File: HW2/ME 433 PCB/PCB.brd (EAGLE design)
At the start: 50 x 50 mm, 22 parts, among them J1 USB-MB-H

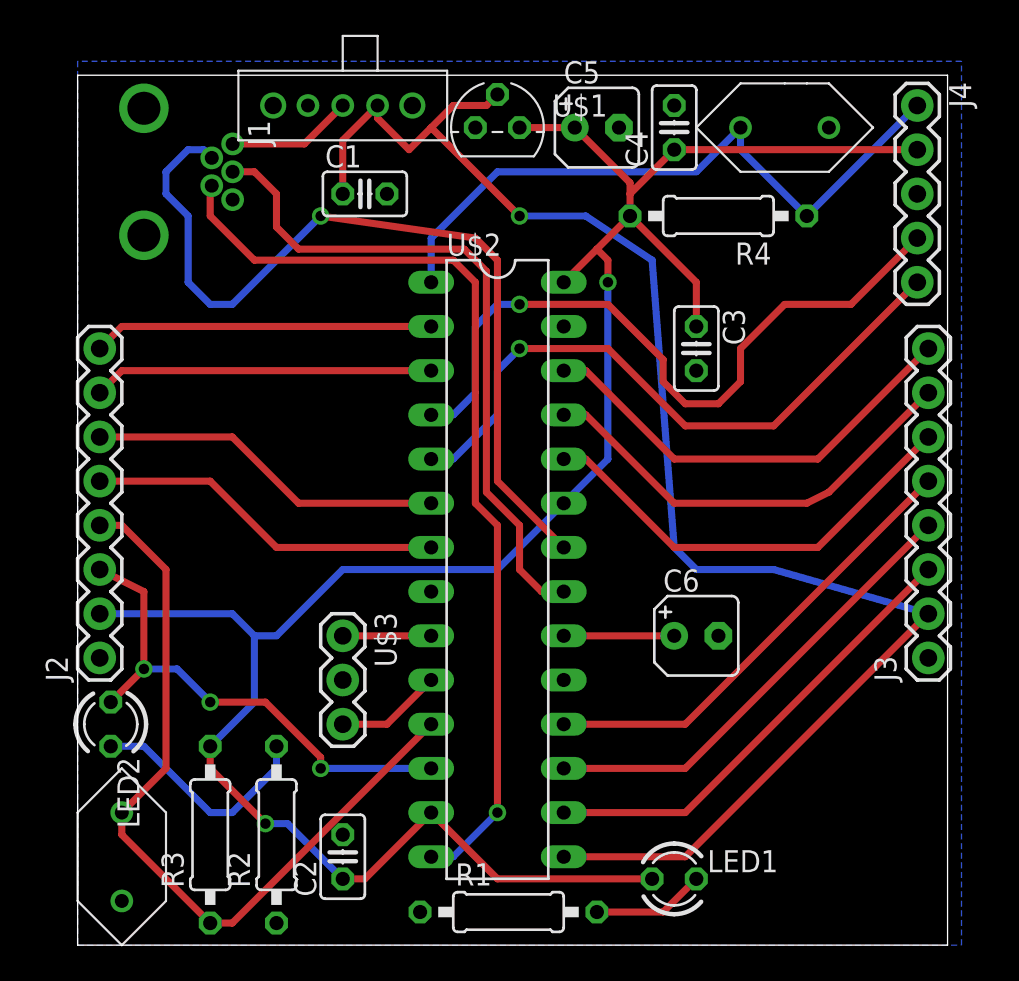
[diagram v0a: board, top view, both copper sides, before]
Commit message: HW2 update
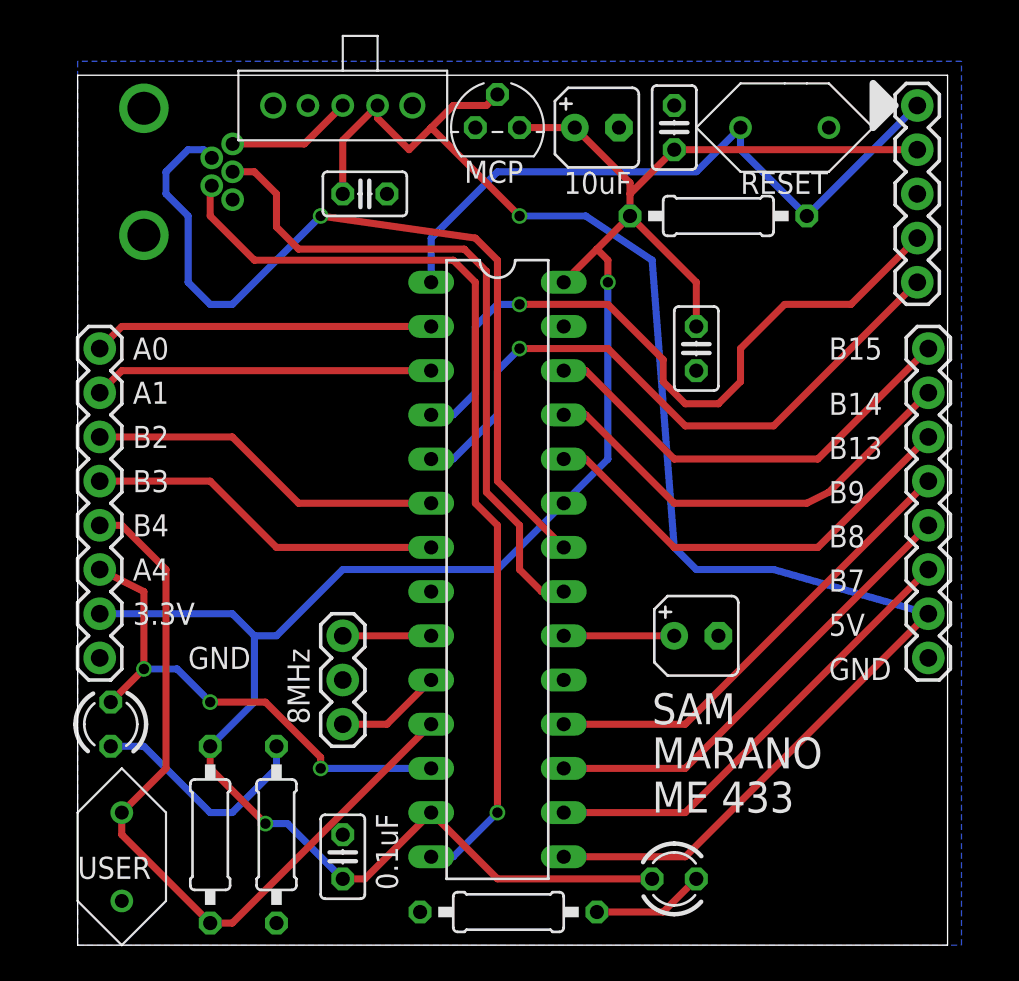
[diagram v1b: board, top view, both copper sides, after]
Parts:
- R3, R4: value (none) -> 10k
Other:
- board text added: "0.1uF"
- board text added: "10uF"
- board text added: "3.3V"
- board text added: "5V"
- board text added: "8MHz"
- board text added: "A0"
- board text added: "A1"
- board text added: "A4"
- board text added: "B13"
- board text added: "B14"
- board text added: "B15"
- board text added: "B2"
- board text added: "B3"
- board text added: "B4"
- board text added: "B7"
- board text added: "B8"
- board text added: "B9"
- board text added: "GND"
- board text added: "MARANO"
- board text added: "MCP"
- board text added: "ME 433"
- board text added: "RESET"
- board text added: "SAM"
- board text added: "USER"
